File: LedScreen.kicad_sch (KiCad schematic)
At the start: 28 parts, among them U1 Teensy4.1, U2 74HCT245

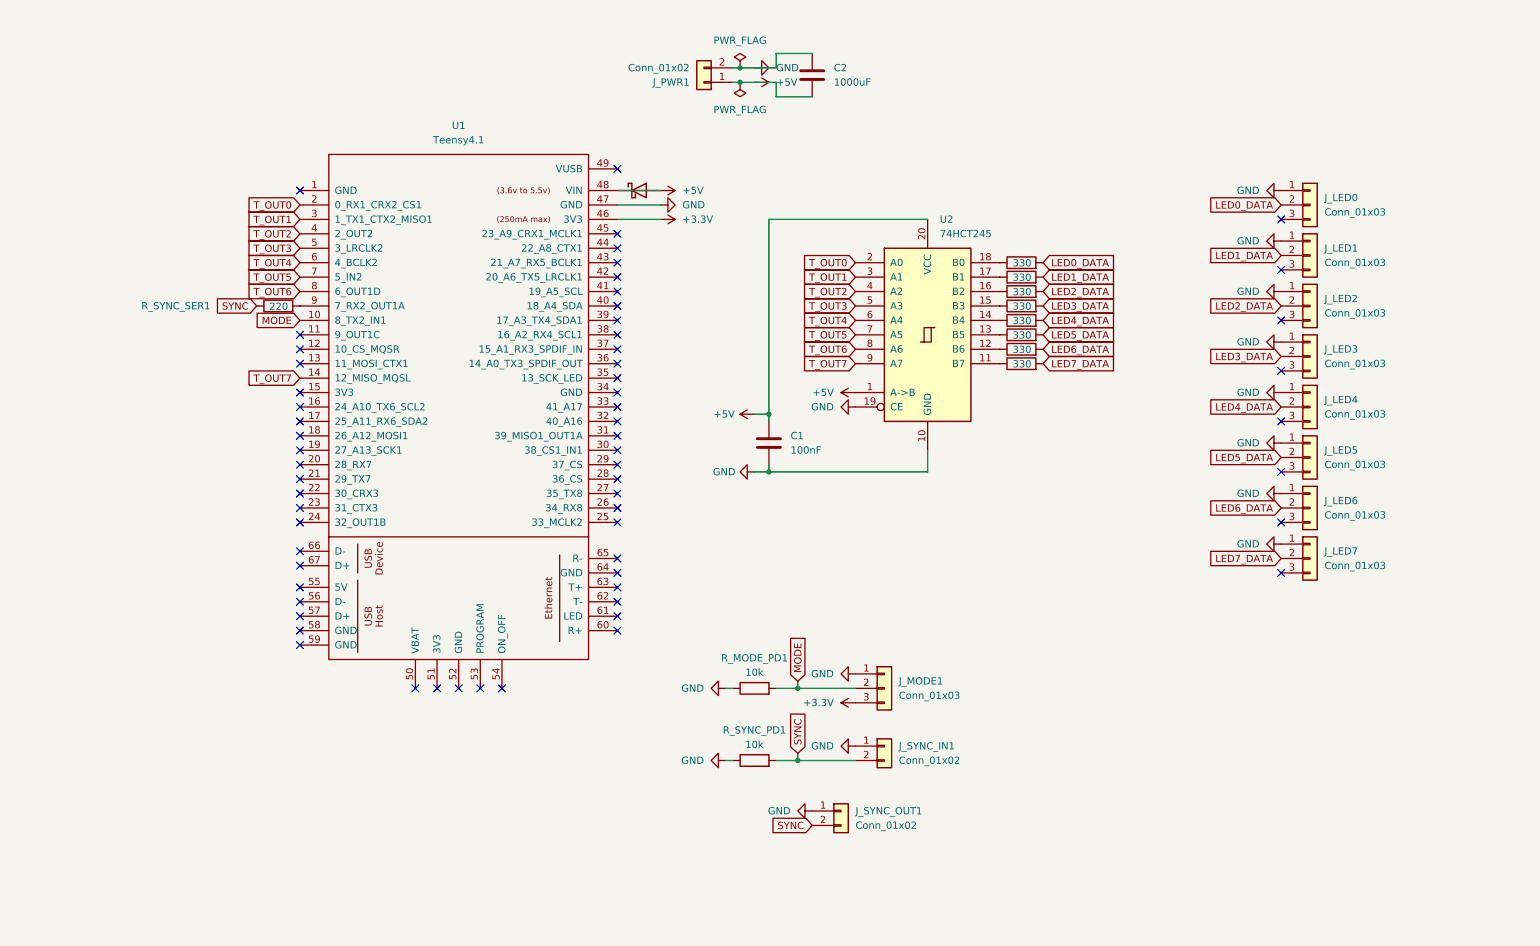
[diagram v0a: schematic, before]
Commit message: DONE WIRINg
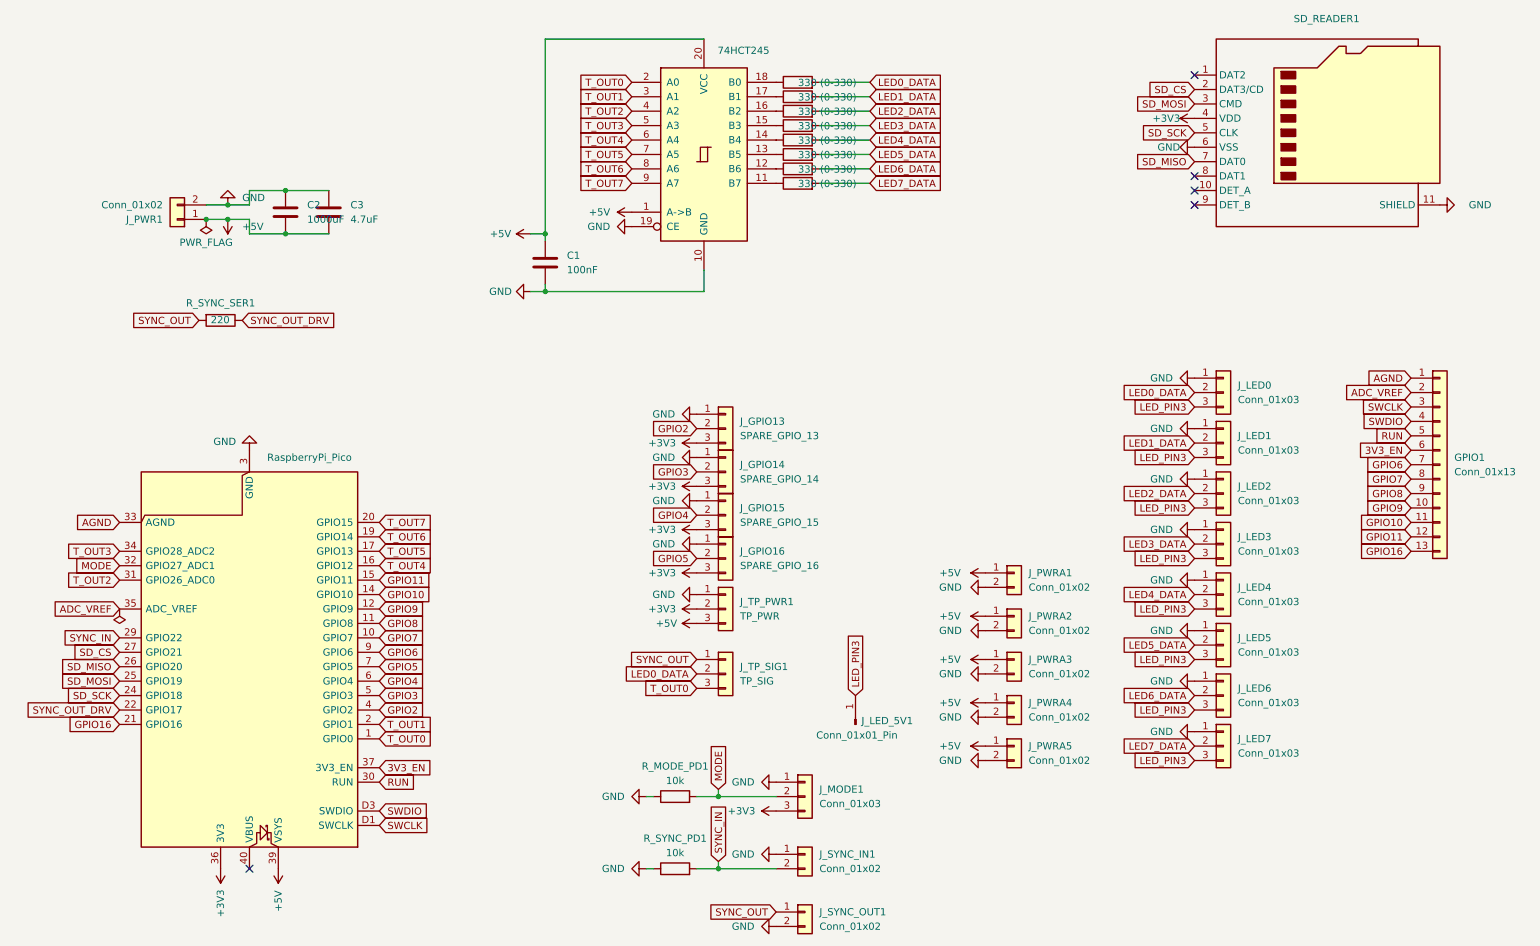
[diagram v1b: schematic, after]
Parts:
- removed D1: D_Schottky, symbol Device:D_Schottky
- removed U1: Teensy4.1, teensy:Teensy41, symbol teensy_library:Teensy4.1
- added A1: RaspberryPi_Pico, Module:RaspberryPi_Pico_SMD_HandSolder, symbol MCU_Module:RaspberryPi_Pico_Debug
- added C3: 4.7uF, Capacitor_SMD:C_1206_3216Metric, symbol Device:C
- added GPIO1: Conn_01x13, Connector_PinHeader_2.54mm:PinHeader_1x13_P2.54mm_Vertical, symbol Connector_Generic:Conn_01x13
- added J_GPIO13: SPARE_GPIO_13, Connector_PinHeader_2.54mm:PinHeader_1x03_P2.54mm_Horizontal, symbol Connector_Generic:Conn_01x03
- added J_GPIO14: SPARE_GPIO_14, Connector_PinHeader_2.54mm:PinHeader_1x03_P2.54mm_Horizontal, symbol Connector_Generic:Conn_01x03
- added J_GPIO15: SPARE_GPIO_15, Connector_PinHeader_2.54mm:PinHeader_1x03_P2.54mm_Horizontal, symbol Connector_Generic:Conn_01x03
- added J_GPIO16: SPARE_GPIO_16, Connector_PinHeader_2.54mm:PinHeader_1x03_P2.54mm_Horizontal, symbol Connector_Generic:Conn_01x03
- added J_LED_5V1: Conn_01x01_Pin, Connector_PinHeader_1.00mm:PinHeader_1x01_P1.00mm_Vertical, symbol Connector:Conn_01x01_Pin
- added J_PWRA1, J_PWRA2, J_PWRA3, J_PWRA4, J_PWRA5: Conn_01x02, Connector_PinHeader_2.54mm:PinHeader_1x02_P2.54mm_Horizontal, symbol Connector_Generic:Conn_01x02
- added J_TP_PWR1: TP_PWR, Connector_PinHeader_2.54mm:PinHeader_1x03_P2.54mm_Horizontal, symbol Connector_Generic:Conn_01x03
- added J_TP_SIG1: TP_SIG, Connector_PinHeader_2.54mm:PinHeader_1x03_P2.54mm_Horizontal, symbol Connector_Generic:Conn_01x03
- added SD_READER1: Micro_SD_Card_Det_Hirose_DM3AT, Connector_Card:microSD_HC_Hirose_DM3AT-SF-PEJM5, symbol Connector:Micro_SD_Card_Det_Hirose_DM3AT
- 74HCT245: renamed from U2; footprint (none) -> Package_DIP:DIP-20_W7.62mm
- C1: footprint (none) -> Capacitor_SMD:C_0805_2012Metric
- C2: footprint (none) -> Capacitor_THT:CP_Radial_D10.0mm_P5.00mm
- J_LED0, J_LED1, J_LED2, J_LED3, J_LED4, J_LED5, J_LED6, J_LED7: footprint (none) -> Connector_PinHeader_2.54mm:PinHeader_1x03_P2.54mm_Horizontal
- J_MODE1: footprint (none) -> Connector_PinHeader_2.54mm:PinHeader_1x03_P2.54mm_Vertical
- J_PWR1, J_SYNC_IN1, J_SYNC_OUT1: footprint (none) -> Connector_PinHeader_2.54mm:PinHeader_1x02_P2.54mm_Horizontal
- R1, R2, R3, R4, R5, R6, R7, R8: value 330 -> 330 (0-330); footprint (none) -> Resistor_SMD:R_0805_2012Metric
- R_MODE_PD1, R_SYNC_PD1, R_SYNC_SER1: footprint (none) -> Resistor_SMD:R_0805_2012Metric
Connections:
- net +5V: now also A1.39 (VSYS), C3.2, J_PWRA1.1 (Pin_1), J_PWRA2.1 (Pin_1), J_PWRA3.1 (Pin_1), J_PWRA4.1 (Pin_1), J_PWRA5.1 (Pin_1), J_TP_PWR1.3 (Pin_3)
- net GND: now also J_SYNC_OUT1.2 (Pin_2), A1.13 (GND), A1.18 (GND), A1.23 (GND), A1.28 (GND), A1.3 (GND), A1.38 (GND), A1.8 (GND), A1.D2 (GND), C3.1, J_GPIO13.1 (Pin_1), J_GPIO14.1 (Pin_1), J_GPIO15.1 (Pin_1), J_GPIO16.1 (Pin_1), J_PWRA1.2 (Pin_2), J_PWRA2.2 (Pin_2), J_PWRA3.2 (Pin_2), J_PWRA4.2 (Pin_2), J_PWRA5.2 (Pin_2), J_TP_PWR1.1 (Pin_1), SD_READER1.11 (SHIELD), SD_READER1.6 (VSS); no longer J_SYNC_OUT1.1 (Pin_1)
- net LED0_DATA: now also J_TP_SIG1.2 (Pin_2)
- net MODE: now also A1.32 (GPIO27_ADC1)
- net T_OUT0: now also A1.1 (GPIO0), J_TP_SIG1.3 (Pin_3)
- net T_OUT1: now also A1.2 (GPIO1)
- net T_OUT2: now also A1.31 (GPIO26_ADC0)
- net T_OUT3: now also A1.34 (GPIO28_ADC2)
- net T_OUT4: now also A1.16 (GPIO12)
- net T_OUT5: now also A1.17 (GPIO13)
- net T_OUT6: now also A1.19 (GPIO14)
- net T_OUT7: now also A1.20 (GPIO15)
- net LED_PIN3: now reaches J_LED6.3 (Pin_3)
- net LED_PIN3: now also J_LED0.3 (Pin_3), J_LED1.3 (Pin_3), J_LED2.3 (Pin_3), J_LED3.3 (Pin_3), J_LED4.3 (Pin_3), J_LED5.3 (Pin_3), J_LED7.3 (Pin_3), J_LED_5V1.1 (Pin_1)
- net SYNC_OUT: now reaches R_SYNC_SER1.2
- net SYNC_OUT: now also J_SYNC_OUT1.1 (Pin_1), J_TP_SIG1.1 (Pin_1)
- net +3.3V renamed +3V3
- net +3V3: now also A1.36 (3V3), J_GPIO13.3 (Pin_3), J_GPIO14.3 (Pin_3), J_GPIO15.3 (Pin_3), J_GPIO16.3 (Pin_3), J_TP_PWR1.2 (Pin_2), SD_READER1.4 (VDD)
- net SYNC renamed SYNC_IN
- net SYNC_IN: now also A1.29 (GPIO22); no longer J_SYNC_OUT1.2 (Pin_2), R_SYNC_SER1.1
- new net 3V3_EN: A1.37 (3V3_EN), GPIO1.6 (Pin_6)
- new net ADC_VREF: A1.35 (ADC_VREF), GPIO1.2 (Pin_2)
- new net AGND: A1.33 (AGND), GPIO1.1 (Pin_1)
- new net GPIO10: A1.14 (GPIO10), GPIO1.11 (Pin_11)
- new net GPIO11: A1.15 (GPIO11), GPIO1.12 (Pin_12)
- new net GPIO16: A1.21 (GPIO16), GPIO1.13 (Pin_13)
- new net GPIO2: A1.4 (GPIO2), J_GPIO13.2 (Pin_2)
- new net GPIO3: A1.5 (GPIO3), J_GPIO14.2 (Pin_2)
- new net GPIO4: A1.6 (GPIO4), J_GPIO15.2 (Pin_2)
- new net GPIO5: A1.7 (GPIO5), J_GPIO16.2 (Pin_2)
- new net GPIO6: A1.9 (GPIO6), GPIO1.7 (Pin_7)
- new net GPIO7: A1.10 (GPIO7), GPIO1.8 (Pin_8)
- new net GPIO8: A1.11 (GPIO8), GPIO1.9 (Pin_9)
- new net GPIO9: A1.12 (GPIO9), GPIO1.10 (Pin_10)
- new net RUN: A1.30 (RUN), GPIO1.5 (Pin_5)
- new net SD_CS: A1.27 (GPIO21), SD_READER1.2 (DAT3/CD)
- new net SD_MISO: A1.26 (GPIO20), SD_READER1.7 (DAT0)
- new net SD_MOSI: A1.25 (GPIO19), SD_READER1.3 (CMD)
- new net SD_SCK: A1.24 (GPIO18), SD_READER1.5 (CLK)
- new net SWCLK: A1.D1 (SWCLK), GPIO1.3 (Pin_3)
- new net SWDIO: A1.D3 (SWDIO), GPIO1.4 (Pin_4)
- new net SYNC_OUT_DRV: A1.22 (GPIO17), R_SYNC_SER1.1
- no-connect marks 62 -> 5
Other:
- company: (none) -> Nick Esselman
- title: (none) -> Led Controler
- moved on the sheet: 74HCT245, C1, C2, J_LED0, J_LED1, J_LED2, J_LED3, J_LED4, J_LED5, J_LED6, J_LED7, J_MODE1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
